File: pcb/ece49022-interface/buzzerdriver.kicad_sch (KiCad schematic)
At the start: 4 parts, among them Q1 C1815

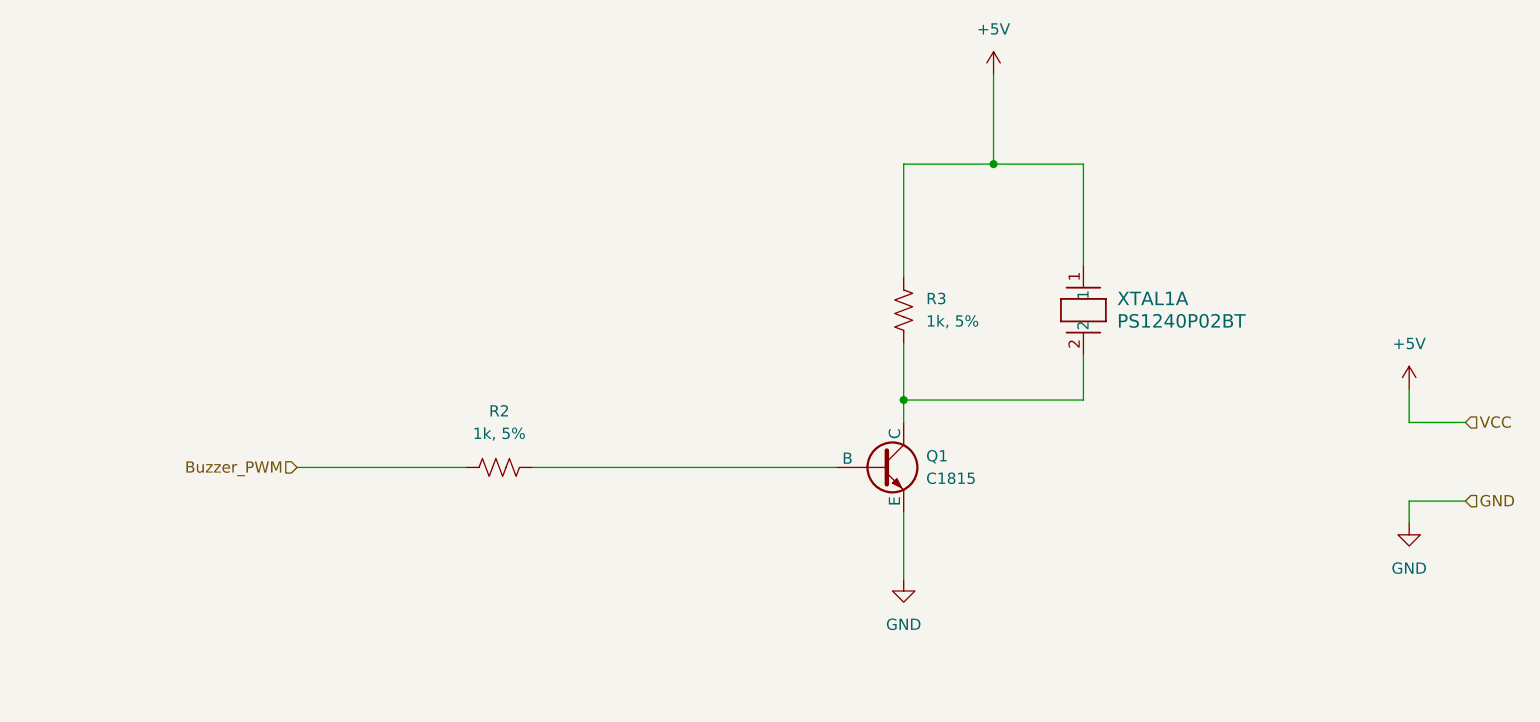
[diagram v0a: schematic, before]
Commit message: Update
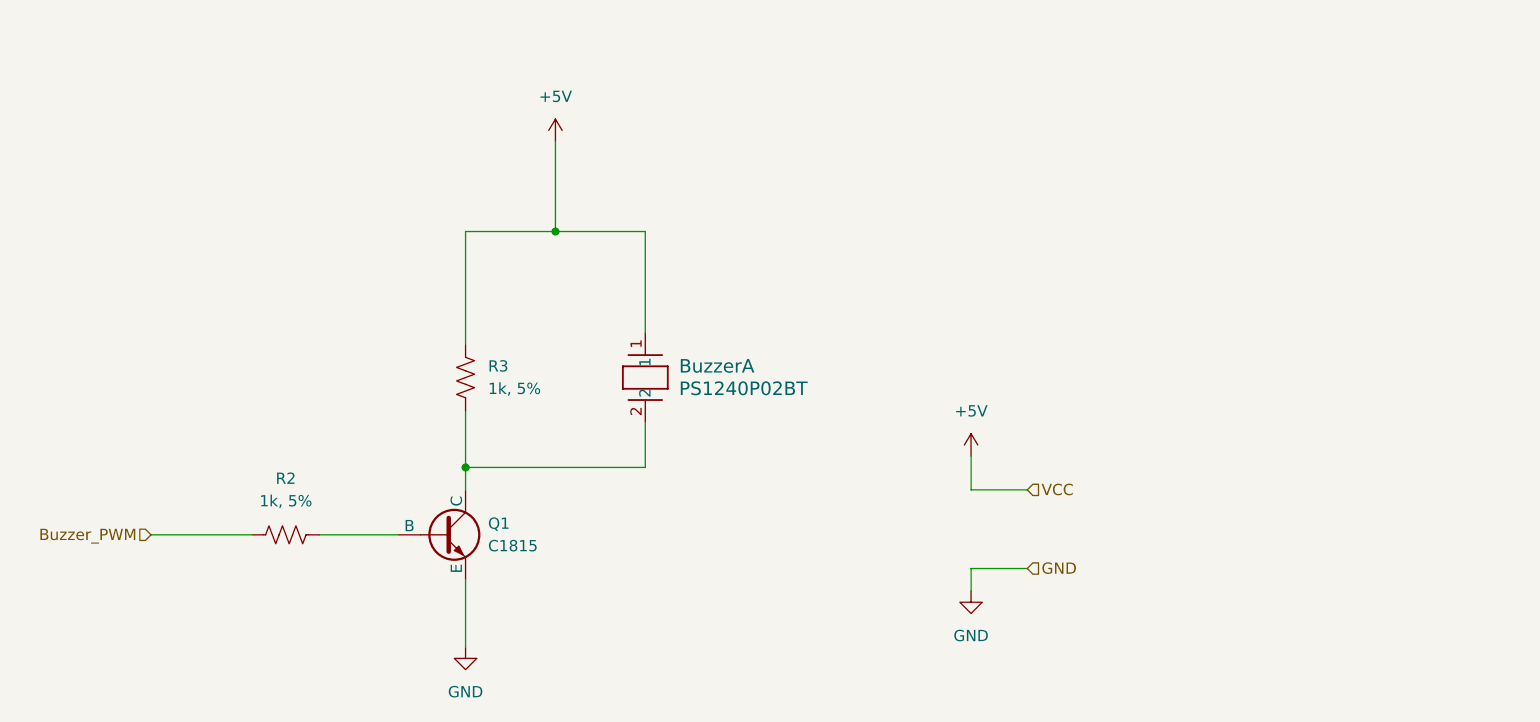
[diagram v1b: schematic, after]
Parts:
- renumbered XTAL1 to Buzzer
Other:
- moved on the sheet: BuzzerA, Q1, R2, R3
